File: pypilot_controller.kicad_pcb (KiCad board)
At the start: 4 copper layers, 76.6 x 50.6 mm, 99 parts, among them J1 power+, J10 Clutch, J2 power-, J3 Motor A, J4 Motor B, J5 UART_Device, J6 Rudder, J7 End Stops, J8 Conn_01x02, J9 ISP, Q1 Q_NMOS_GDS, Q2 Q_NMOS_GDS, Q3 Q_NMOS_GDS, Q4 Q_NMOS_GDS, Q5 Q_NMOS_GDS, T1 Tooling, T2 Tooling, T3 Tooling, U1 SN74LVC1G17DBVR, U10 TLP2361(TPL,E(T, U2 IR2101, U3 IR2101, U4 XC6202P502FR-G, U5 SN74LVC1G17DBVR, U6 LM317, U7 ATmega328P-AU, U8 SN74LVC1G17DBVR, U9 TLP2361(TPL,E(T, Y1 8mhz

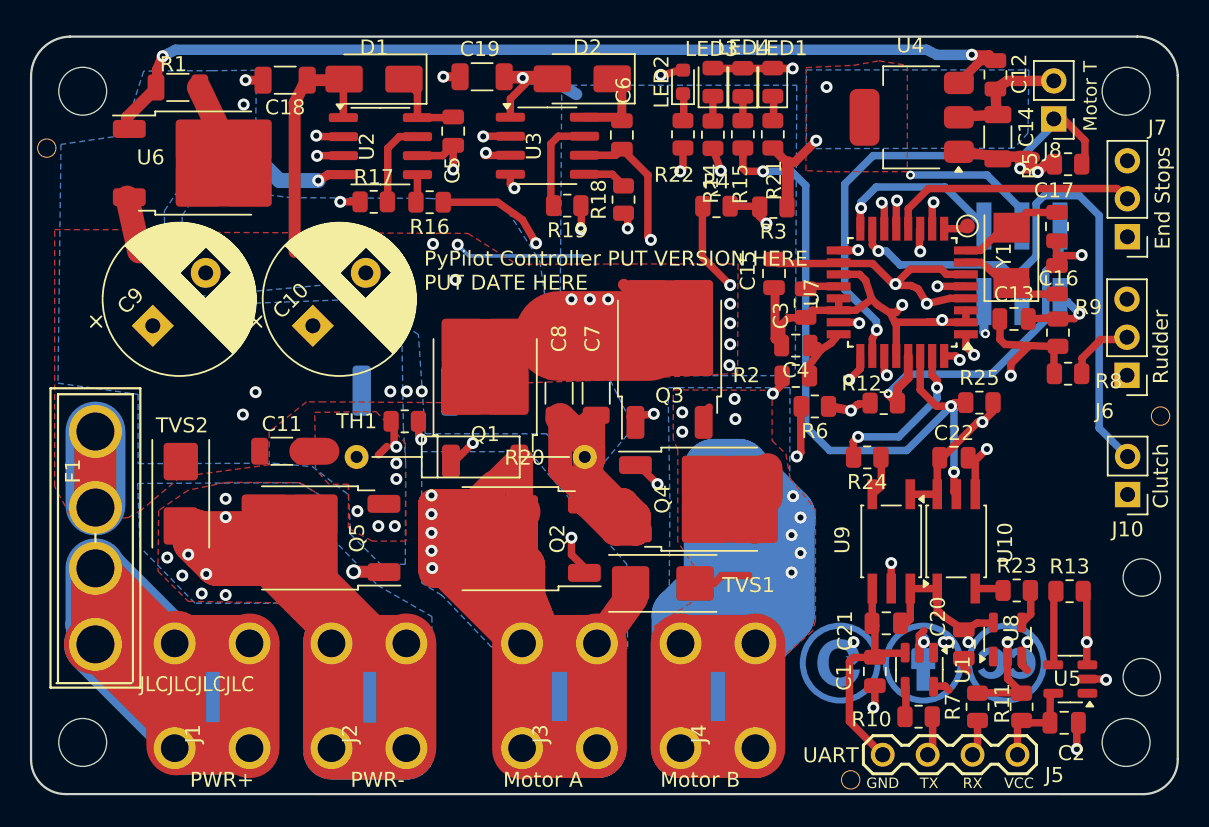
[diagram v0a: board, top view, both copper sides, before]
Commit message: Cleaned up designators - where possible, they are all right way up
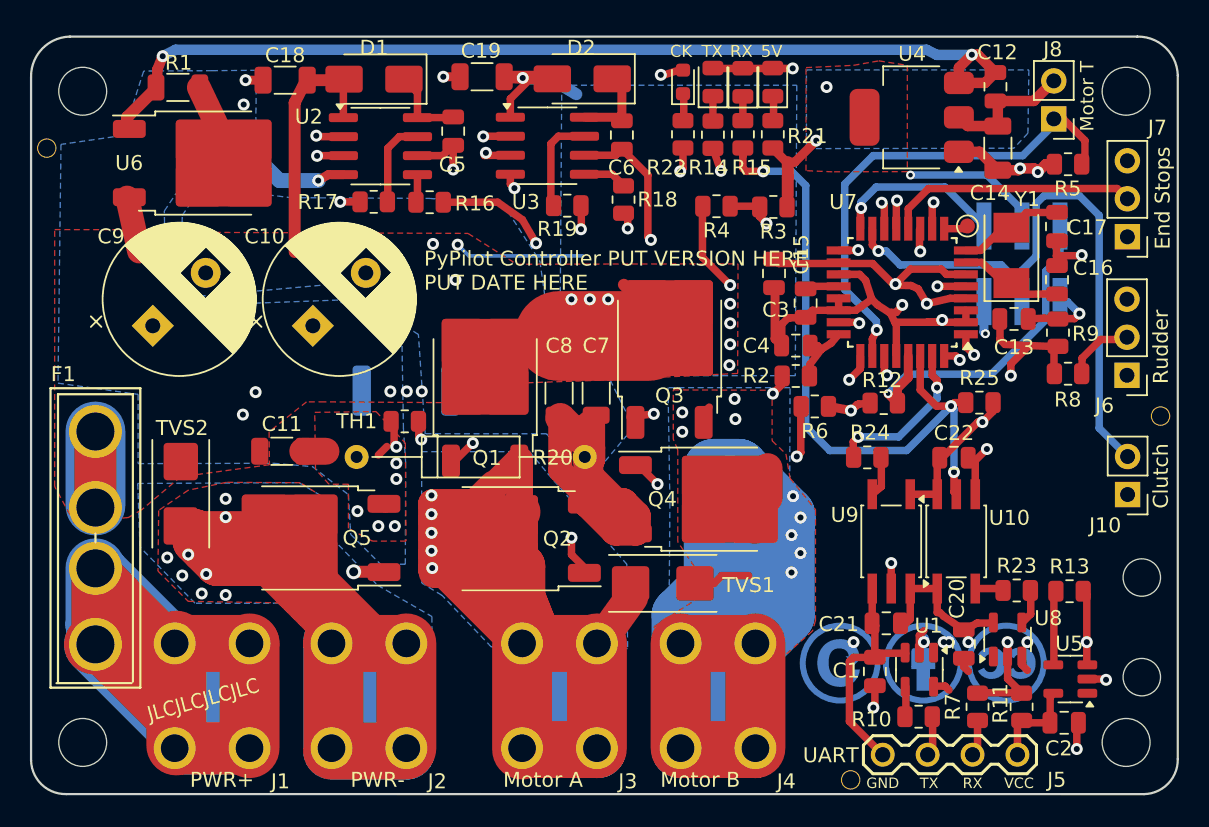
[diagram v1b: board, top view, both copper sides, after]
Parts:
- moved C12 0.79 mm to (66.3, 4.30)
- moved C14 0.76 mm to (66.4, 8.40)
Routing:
- net +5V: track 122.1 -> 118.3 mm
- net Net-(U4-VI): track 65.2 -> 67.1 mm
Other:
- board text added: "5V"
- board text added: "CK"
- board text added: "RX"
- board text added: "TX"
